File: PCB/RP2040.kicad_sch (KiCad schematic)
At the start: 1 part

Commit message: final footprints
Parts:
- U2: footprint Library:Raspberry_pi_pico -> Connector_PinSocket_2.54mm:PinSocket_2x20_P2.54mm_Vertical_SMD
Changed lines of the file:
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@@
 			)
 		)
-		(property "Footprint" "Library:Raspberry_pi_pico"
+		(property "Footprint" "Connector_PinSocket_2.54mm:PinSocket_2x20_P2.54mm_Vertical_SMD"
 			(at 166.37 128.27 0)
 			(effects

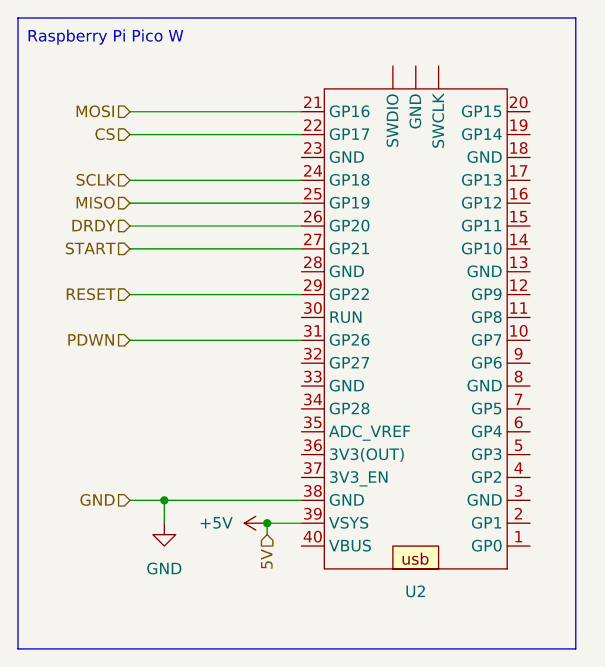
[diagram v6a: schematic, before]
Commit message: initial pcb import
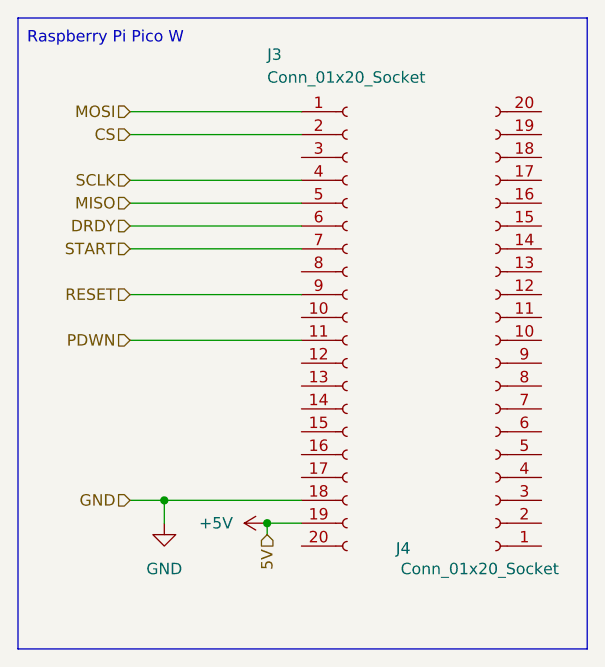
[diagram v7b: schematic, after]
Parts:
- removed U2: ~, Connector_PinSocket_2.54mm:PinSocket_2x20_P2.54mm_Vertical_SMD, symbol custom_lib:pi_pico
- added J3, J4: Conn_01x20_Socket, Connector_PinSocket_2.54mm:PinSocket_1x20_P2.54mm_Vertical, symbol Connector:Conn_01x20_Socket
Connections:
- net +5V: now also J3.19 (Pin_19)
- net CS: now also J3.2 (Pin_2)
- net DRDY: now also J3.6 (Pin_6)
- net GND: now also J3.18 (Pin_18)
- net MISO: now also J3.5 (Pin_5)
- net MOSI: now also J3.1 (Pin_1)
- net PDWN: now also J3.11 (Pin_11)
- net RESET: now also J3.9 (Pin_9)
- net SCLK: now also J3.4 (Pin_4)
- net START: now also J3.7 (Pin_7)
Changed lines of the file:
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@@
 	(rectangle
 		(start 122.174 64.516)
-		(end 184.15 134.62)
+		(end 185.42 134.62)
 		(stroke
 			(width 0)
@@
 	)
 	(symbol
-		(lib_id "custom_lib:pi_pico")
-		(at 166.37 128.27 180)
+		(lib_id "Connector:Conn_01x20_Socket")
+		(at 175.26 100.33 180)
 		(unit 1)
 		(exclude_from_sim no)
@@
 		(on_board yes)
 		(dnp no)
-		(fields_autoplaced yes)
-		(property "Reference" "U2"
-			(at 166.37 128.27 0)
-			(effects
-				(font
-					(size 1.27 1.27)
-				)
-			)
-		)
-		(property "Value" "~"
-			(at 166.37 129.54 0)
-			(effects
-				(font
-					(size 1.27 1.27)
-				)
-			)
-		)
-		(property "Footprint" "Connector_PinSocket_2.54mm:PinSocket_2x20_P2.54mm_Vertical_SMD"
-			(at 166.37 128.27 0)
-			(effects
-				(font
-					(size 1.27 1.27)
-				)
-				(hide yes)
-			)
-		)
-		(property "Datasheet" ""
-			(at 166.37 128.27 0)
-			(effects
-				(font
-					(size 1.27 1.27)
-				)
-				(hide yes)
-			)
-		)
-		(property "Description" ""
-			(at 166.37 128.27 0)
-			(effects
-				(font
-					(size 1.27 1.27)
-				)
-				(hide yes)
-			)
+		(property "Reference" "J4"
+			(at 164.973 123.444 0)
+			(effects
+				(font
+					(size 1.27 1.27)
+				)
+			)
+		)
+		(property "Value" "Conn_01x20_Socket"
+			(at 173.482 125.73 0)
+			(effects
+				(font
+					(size 1.27 1.27)
+				)
+			)
+		)
+		(property "Footprint" "Connector_PinSocket_2.54mm:PinSocket_1x20_P2.54mm_Vertical"
+			(at 175.26 100.33 0)
+			(effects
+				(font
+					(size 1.27 1.27)
+				)
+				(hide yes)
+			)
+		)
+		(property "Datasheet" "~"
+			(at 175.26 100.33 0)
+			(effects
+				(font
+					(size 1.27 1.27)
+				)
+				(hide yes)
+			)
+		)
+		(property "Description" "Generic connector, single row, 01x20, script generated"
+			(at 175.26 100.33 0)
+			(effects
+				(font
+					(size 1.27 1.27)
+				)
+				(hide yes)
+			)
+		)
+		(pin "13"
+		)
+		(pin "9"
+		)
+		(pin "1"
+		)
+		(pin "3"
+		)
+		(pin "4"
+		)
+		(pin "15"
+		)
+		(pin "12"
 		)
 		(pin "10"
 		)
-		(pin "22"
-		)
-		(pin "23"
-		)
-		(pin "34"
-		)
-		(pin "26"
-		)
-		(pin "31"
+		(pin "2"
+		)
+		(pin "6"
+		)
+		(pin "7"
+		)
+		(pin "5"
+		)
+		(pin "16"
+		)
+		(pin "19"
+		)
+		(pin "11"
 		)
 		(pin "20"
 		)
-		(pin "16"
-		)
-		(pin "25"
-		)
-		(pin "24"
-		)
-		(pin "11"
-		)
-		(pin "21"
-		)
-		(pin "27"
-		)
-		(pin "29"
-		)
-		(pin "13"
+		(pin "18"
+		)
+		(pin "17"
+		)
+		(pin "8"
 		)
 		(pin "14"
-		)
-		(pin "28"
-		)
-		(pin "3"
-		)
-		(pin "19"
-		)
-		(pin "18"
-		)
-		(pin "30"
-		)
-		(pin "32"
-		)
-		(pin "12"
-		)
-		(pin "33"
-		)
-		(pin "17"
-		)
-		(pin "15"
-		)
-		(pin "35"
-		)
-		(pin "39"
-		)
-		(pin "4"
-		)
-		(pin "37"
-		)
-		(pin ""
-		)
-		(pin ""
-		)
-		(pin "6"
-		)
-		(pin "1"
-		)
-		(pin "7"
-		)
-		(pin "38"
-		)
-		(pin "8"
-		)
-		(pin ""
-		)
-		(pin "36"
-		)
-		(pin "5"
-		)
-		(pin "9"
-		)
-		(pin "40"
-		)
-		(pin "2"
 		)
 		(instances
 			(project "PCBs"
 				(path "/5beccadf-d27e-4f5e-8faf-404ef06d8def/3292d6ff-aa18-48ee-9b41-06ae4ff9c070"
-					(reference "U2")
+					(reference "J4")
 					(unit 1)
 				)
@@
 					(unit 1)
 				)
+			)
+		)
+	)
+	(symbol
+		(lib_id "Connector:Conn_01x20_Socket")
+		(at 158.75 97.79 0)
+		(unit 1)
+		(exclude_from_sim no)
+		(in_bom yes)
+		(on_board yes)
+		(dnp no)
+		(property "Reference" "J3"
+			(at 149.86 68.58 0)
+			(effects
+				(font
+					(size 1.27 1.27)
+				)
+				(justify left)
+			)
+		)
+		(property "Value" "Conn_01x20_Socket"
+			(at 149.86 71.12 0)
+			(effects
+				(font
+					(size 1.27 1.27)
+				)
+				(justify left)
+			)
+		)
+		(property "Footprint" "Connector_PinSocket_2.54mm:PinSocket_1x20_P2.54mm_Vertical"
+			(at 158.75 97.79 0)
+			(effects
+				(font
+					(size 1.27 1.27)
+				)
+				(hide yes)
+			)
+		)
+		(property "Datasheet" "~"
+			(at 158.75 97.79 0)
+			(effects
+				(font
+					(size 1.27 1.27)
+				)
+				(hide yes)
+			)
+		)
+		(property "Description" "Generic connector, single row, 01x20, script generated"
+			(at 158.75 97.79 0)
+			(effects
+				(font
+					(size 1.27 1.27)
+				)
+				(hide yes)
+			)
+		)
+		(pin "13"
+		)
+		(pin "9"
+		)
+		(pin "1"
+		)
+		(pin "3"
+		)
+		(pin "4"
+		)
+		(pin "15"
+		)
+		(pin "12"
+		)
+		(pin "10"
+		)
+		(pin "2"
+		)
+		(pin "6"
+		)
+		(pin "7"
+		)
+		(pin "5"
+		)
+		(pin "16"
+		)
+		(pin "19"
+		)
+		(pin "11"
+		)
+		(pin "20"
+		)
+		(pin "18"
+		)
+		(pin "17"
+		)
+		(pin "8"
+		)
+		(pin "14"
+		)
+		(instances
+			(project ""
+				(path "/5beccadf-d27e-4f5e-8faf-404ef06d8def/3292d6ff-aa18-48ee-9b41-06ae4ff9c070"
+					(reference "J3")
+					(unit 1)
+				)
